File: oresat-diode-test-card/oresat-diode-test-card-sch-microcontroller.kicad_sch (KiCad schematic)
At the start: 25 parts, among them J7 ORESAT-DEBUG-CONNECTOR-ALL, U1 TCAN330, U7 STM32F091C, X2 CRYSTAL-WITH-GND

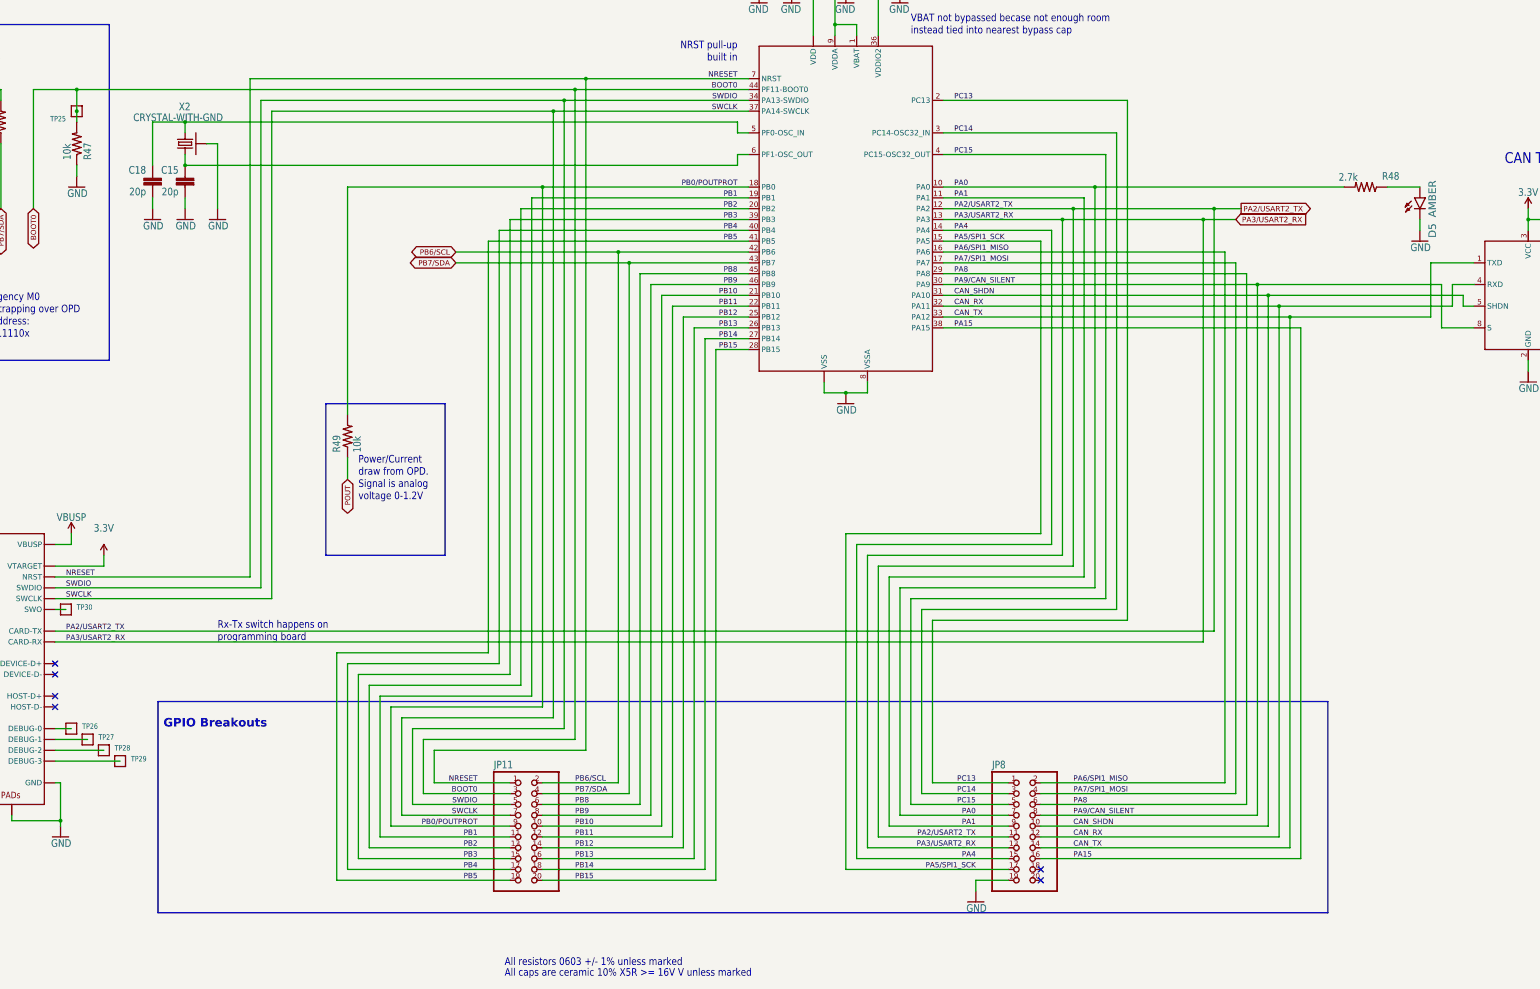
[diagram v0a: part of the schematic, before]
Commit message: added actual files
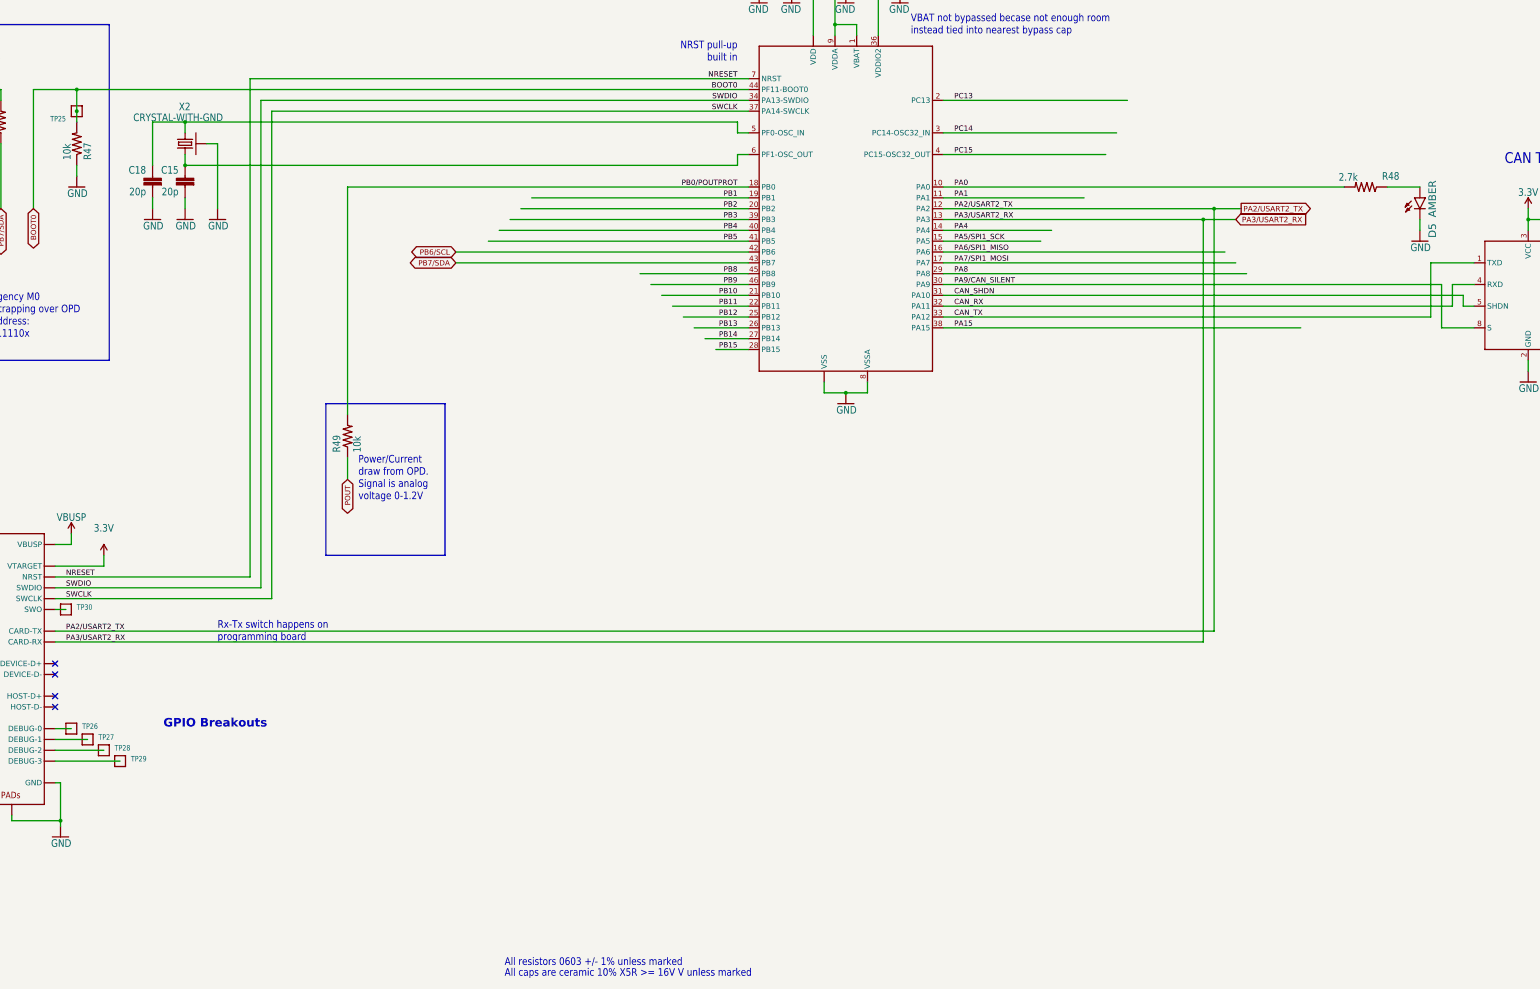
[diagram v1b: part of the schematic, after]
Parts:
- removed JP11, JP8: PINHD-2X10, oresat-proto-card:2X10, symbol oresat-proto-card-eagle-import:PINHD-2X10
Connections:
- no-connect marks 6 -> 4
